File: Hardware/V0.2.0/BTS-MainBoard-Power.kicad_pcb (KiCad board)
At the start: 4 copper layers, 100 x 100 mm, 62 parts, among them J10 PeCon, J11 PeCon, J12 FanConn, J13 FanConn, J14 FanConn, J15 FanConn, J16 FanConn, J17 FanConn, J18 FanConn, J19 FanConn, J3 LogicBoardConnector, J4 PeCon, J5 PeCon, J6 PeCon, J7 PeCon, J8 PeCon, J9 PeCon, Q1 DMG3418L, Q2 NTMFS5H419NL, Q3 NTMFS5H419NL, Q4 NTMFS5H419NL, Q5 NTMFS5H419NL, U1 LM5109BMA, U2 LM5109BMA

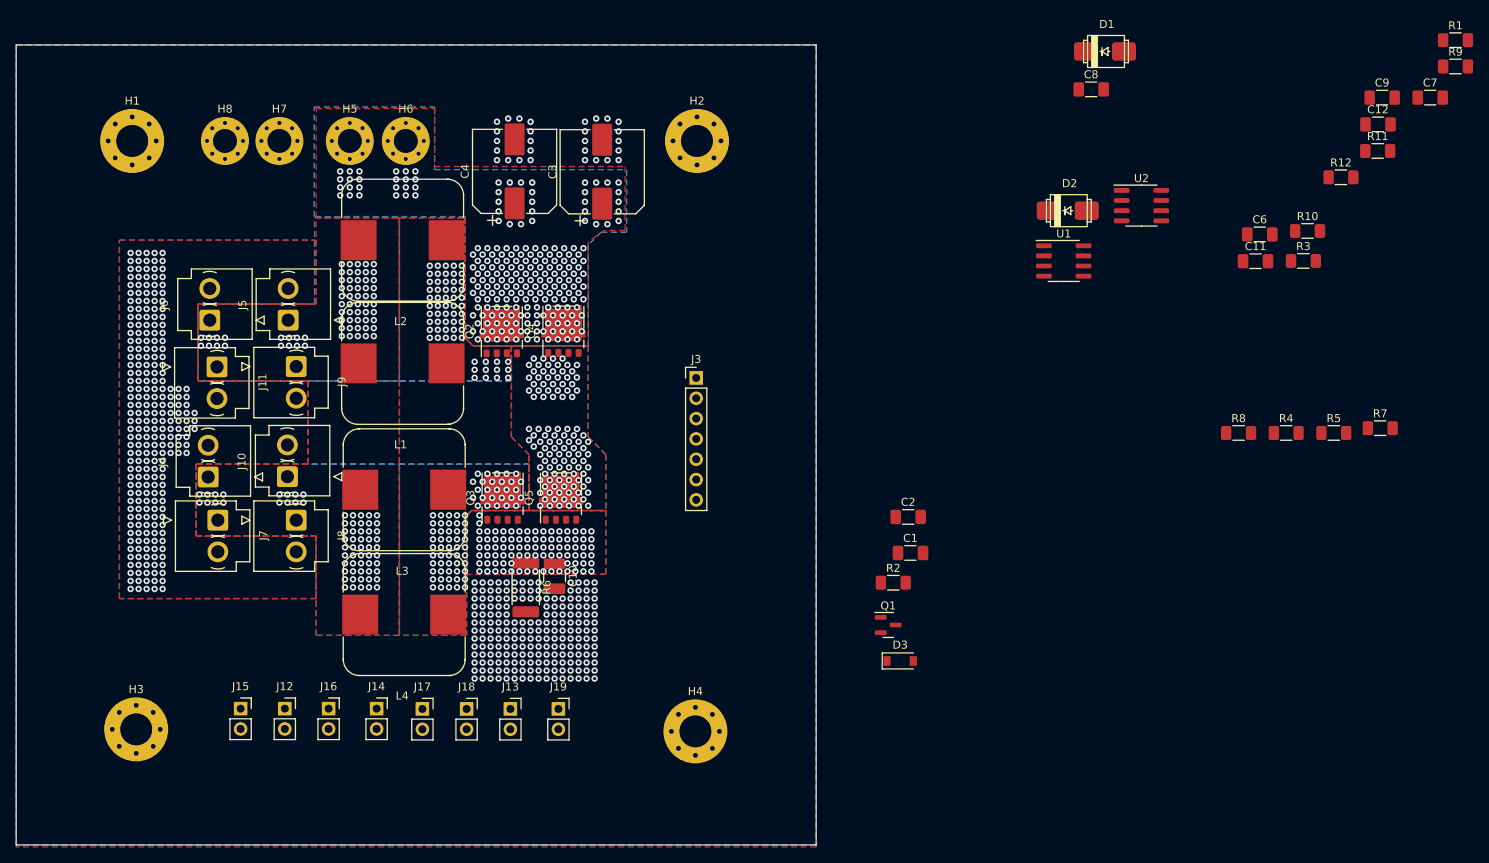
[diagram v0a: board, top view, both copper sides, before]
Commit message: Finished routing, now needs improvements
Signed-off-by: bebenlebricolo <benoittarrade@hotmail.fr>
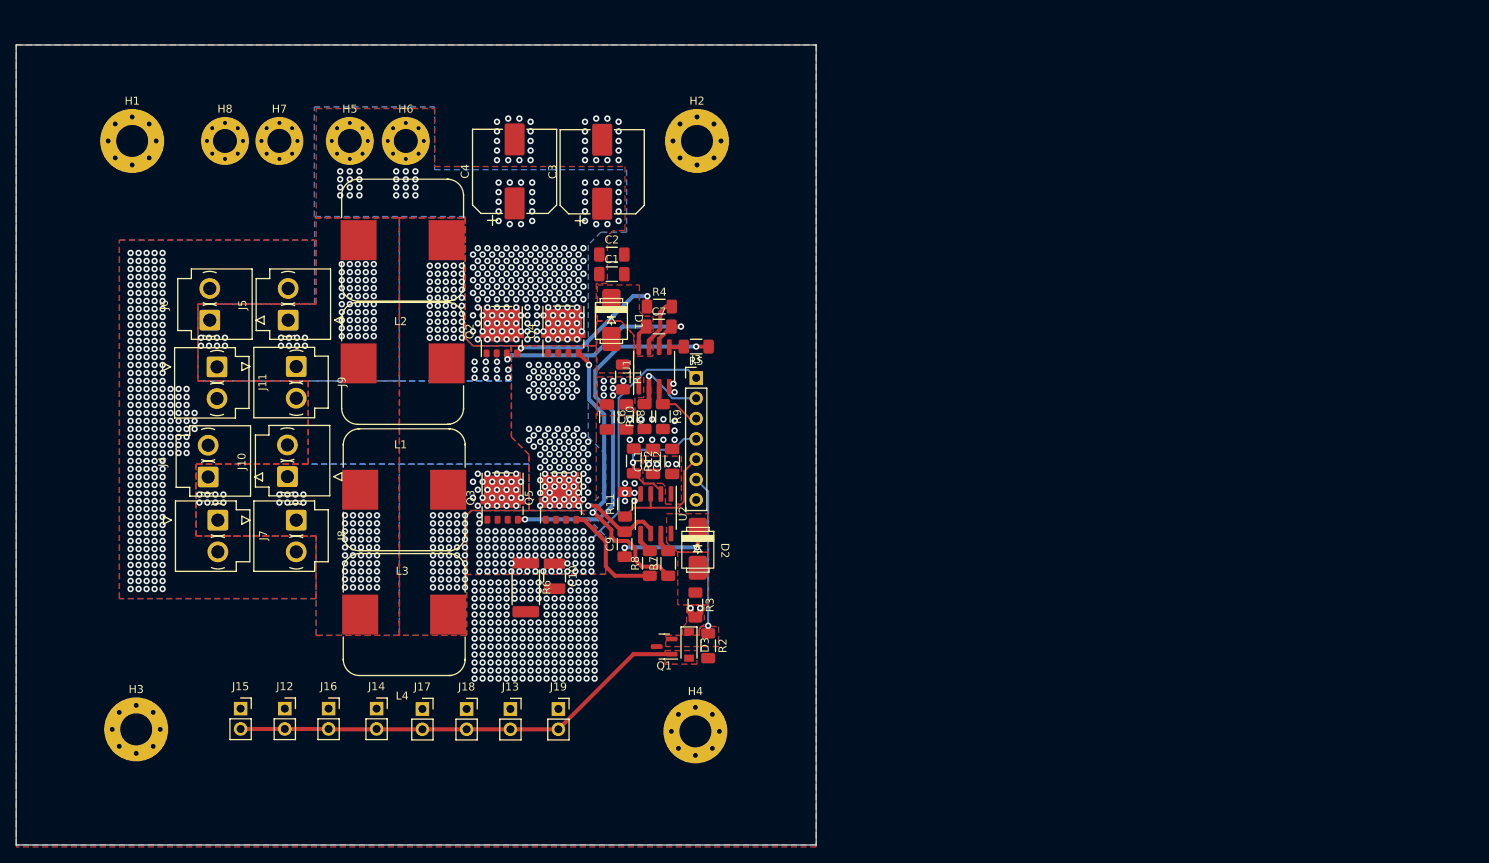
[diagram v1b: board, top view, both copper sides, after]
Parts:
- moved R1 112.3 mm to (174.3, 78.5), turned to -90 degrees
- moved C9 109.9 mm to (174.6, 99.4), turned to 90 degrees
- moved R9 108.3 mm to (179.3, 83.5), turned to -90 degrees
- moved R11 103.9 mm to (174.6, 94.4), turned to 90 degrees
- moved C7 100.6 mm to (178.8, 72.2)
- moved C12 97.8 mm to (180.5, 89.0), turned to 90 degrees
- moved R12 95.2 mm to (175.7, 89.0), turned to -90 degrees
- moved R7 90.6 mm to (180.0, 101.8), turned to 90 degrees
- moved R3 87.3 mm to (183.4, 107.0), turned to -90 degrees
- moved R10 86.1 mm to (177.0, 83.5), turned to 90 degrees
- moved C6 84.7 mm to (172.3, 83.5), turned to -90 degrees
- moved R5 80.4 mm to (183.5, 74.7), turned to 180 degrees
- moved R4 79.9 mm to (178.9, 69.7)
- moved C11 79.4 mm to (178.1, 89.0), turned to 90 degrees
- moved R8 75.4 mm to (177.7, 101.8), turned to 90 degrees
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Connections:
- D3 pad 1: /Vcc -> /Psu12V
- J12 pad 1: /Vcc -> /Psu12V
- J13 pad 1: /Vcc -> /Psu12V
- J14 pad 1: /Vcc -> /Psu12V
- J15 pad 1: /Vcc -> /Psu12V
- J16 pad 1: /Vcc -> /Psu12V
- J17 pad 1: /Vcc -> /Psu12V
- J18 pad 1: /Vcc -> /Psu12V
- J19 pad 1: /Vcc -> /Psu12V
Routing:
- net /FanSink: track 0.00 -> 57.8 mm
- net /HBridge/ALO_Gate: track 0.00 -> 46.0 mm, vias 0 -> 2
- net /HBridge/BHO_Gate: track 0.00 -> 35.9 mm, vias 0 -> 2
- net /VSense: track 0.00 -> 30.7 mm, vias 86 -> 85
- net /AHS: track 0.00 -> 28.6 mm, vias 139 -> 140
- net /CoolingFanDriveSignal: track 0.00 -> 20.8 mm, vias 0 -> 1
- net /HBridge/AHO_Gate: track 0.00 -> 20.7 mm, vias 0 -> 2
- net /BHO_Sig: track 0.00 -> 15.8 mm, vias 0 -> 1
- net /BLO_Sig: track 0.00 -> 15.6 mm
- net /HBridge/BLO_Gate: track 0.00 -> 13.9 mm
- net /HBoot2: track 0.00 -> 12.4 mm, vias 0 -> 2
- net /AHO_Sig: track 0.00 -> 10.9 mm, vias 0 -> 1
- net /BHS: track 0.00 -> 10.6 mm, vias 357 -> 352
- net /ALO_Sig: track 0.00 -> 7.28 mm
- net /AHO: track 0.00 -> 6.69 mm
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- added copper zone on F.Cu, net /CoolingFanDriveSignal
- added copper zone on F.Cu, net /DBootAnode1
- added copper zone on F.Cu, net /DBootAnode2
- added copper zone on F.Cu, net /FanSink
- added copper zone on F.Cu, net /HBoot1
- added copper zone on F.Cu, net /HBoot2
